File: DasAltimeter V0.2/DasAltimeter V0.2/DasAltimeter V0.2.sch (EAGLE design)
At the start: 53 parts, among them IC1 BMI055, U1 ATSAMD21G-A, U2 3.3V/150mA, U3 MS5803-14BA, U4 ADXL193, X1 22-23-2041, X2 22-23-2041

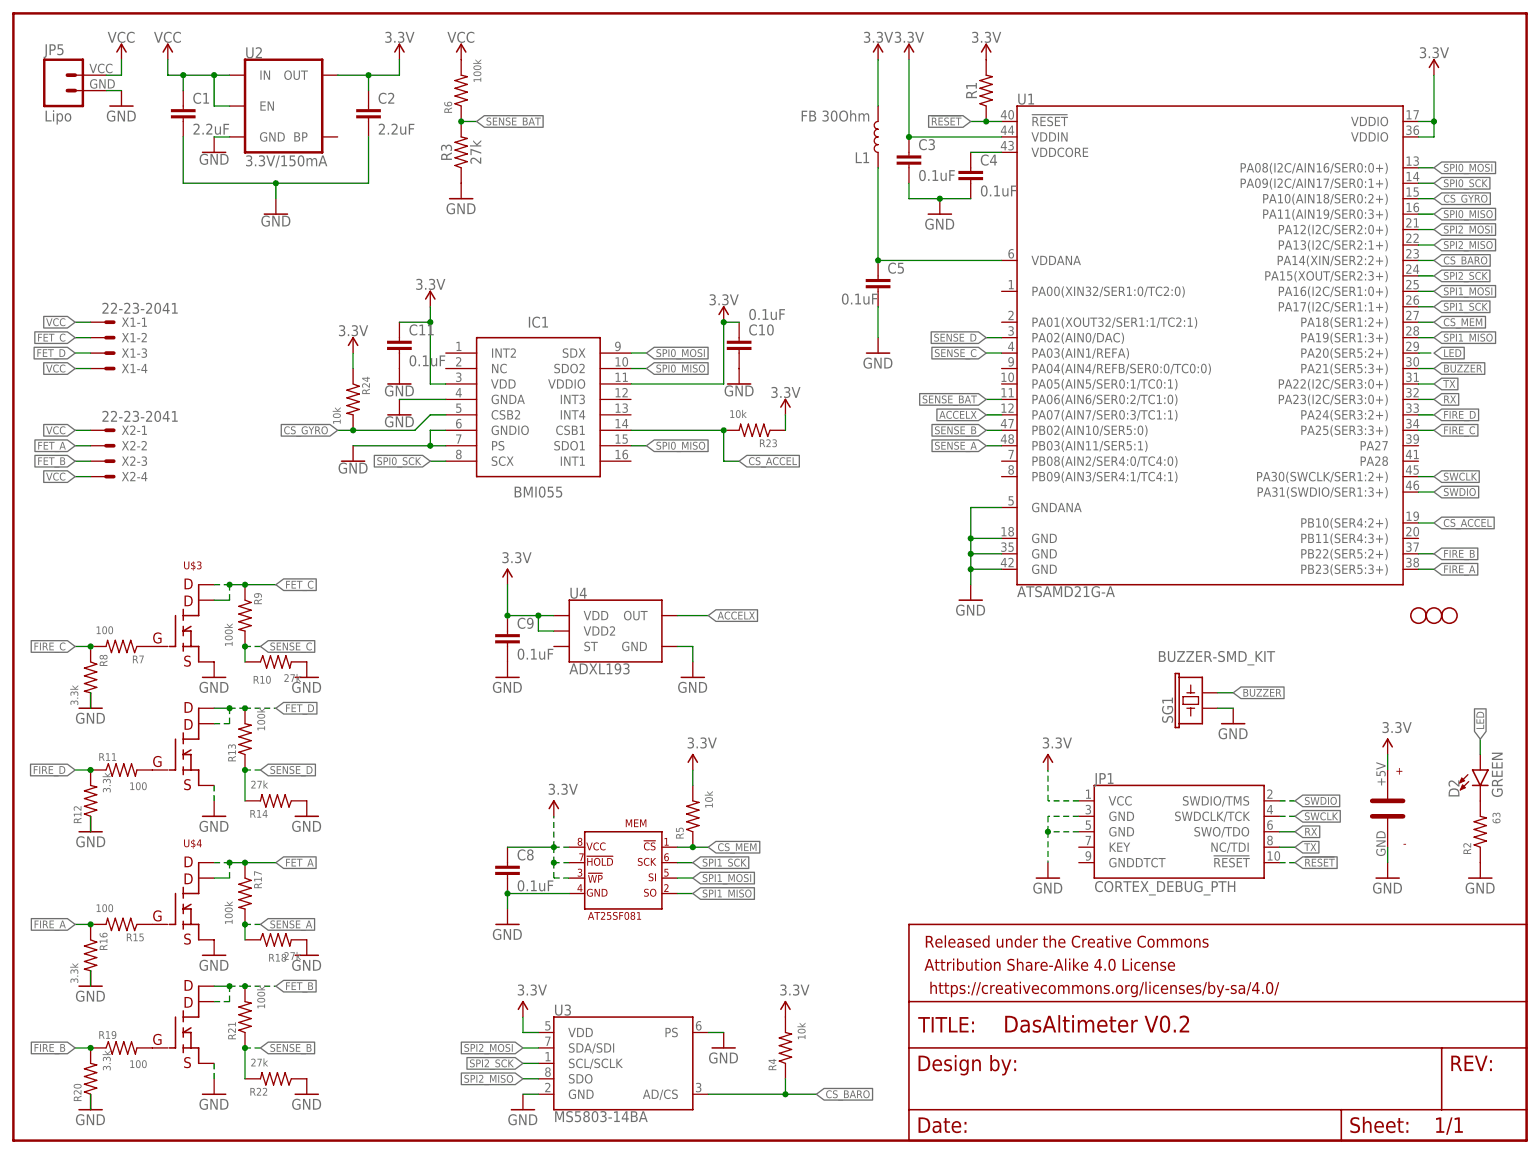
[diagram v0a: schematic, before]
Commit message: playing with mini altimeter idea
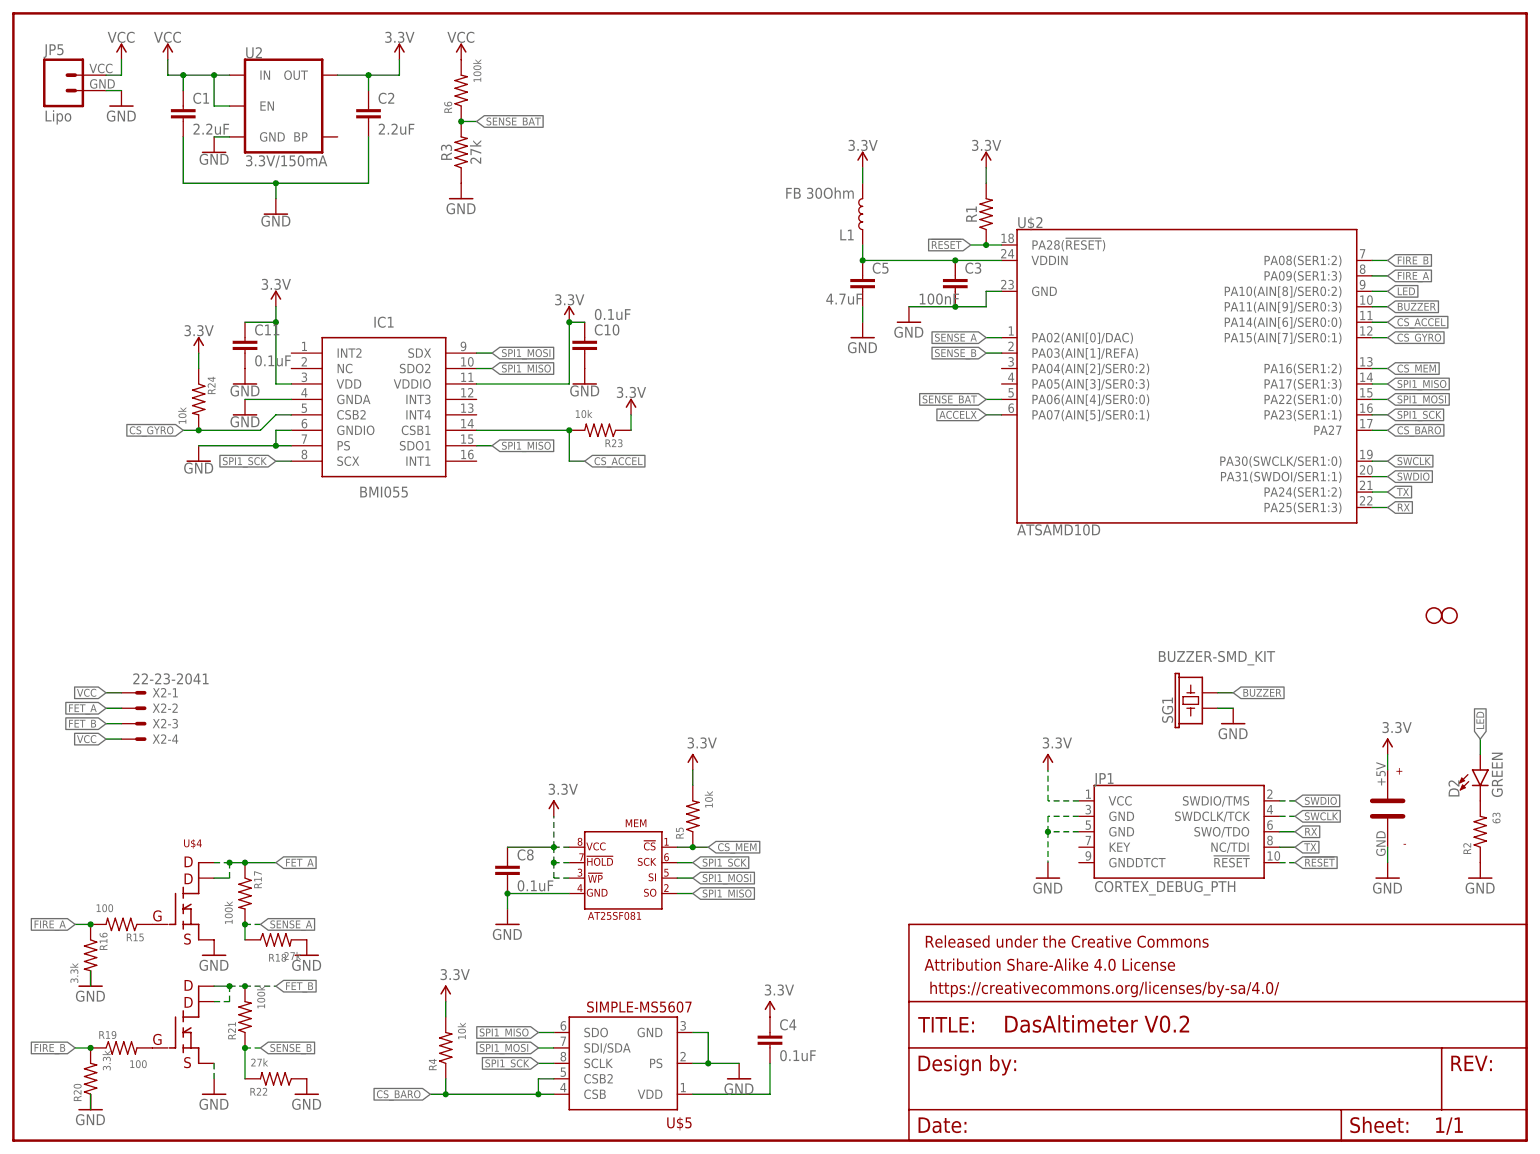
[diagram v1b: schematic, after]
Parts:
- removed C9: 0.1uF, SparkFun-Capacitors:0.1UF-0402-16V-10%
- removed H1: STAND-OFFTIGHT, SparkFun-Hardware:STAND-OFFTIGHT
- removed R10, R14: 27k, SparkFun-Resistors:RESISTOR0402
- removed R11, R7: 100, SparkFun-Resistors:RESISTOR0402
- removed R12, R8: 3.3k, SparkFun-Resistors:RESISTOR0402
- removed R13, R9: 100k, SparkFun-Resistors:RESISTOR0402
- removed U$3: SI7232DN, SaL-lib1:SI7232DN
- removed U1: ATSAMD21G-A, SparkFun-IC-Microcontroller:ATSAMD21G-A
- removed U3: MS5803-14BA, SparkFun-Sensors:MS5803-14BA
- removed U4: ADXL193, SparkFun-Sensors:ADXL193
- removed X1: 22-23-2041, con-molex:22-23-2041
- added U$2: ATSAMD10D, SaL-lib1:ATSAMD10D
- added U$5: SIMPLE-MS5607, MS5607:SIMPLE-MS5607
- C3: value 0.1uF -> 100nF
- C5: value 0.1uF -> 4.7uF
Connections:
- removed net FET_C: R9.1, U$3.PIN7, U$3.PIN8, X1-2.S
- removed net FET_D: R13.2, U$3.PIN5, U$3.PIN6, X1-3.S
- removed net FIRE_C: R7.2, R8.1, U1.PA25(SER3:3+)
- removed net FIRE_D: R11.1, R12.2, U1.PA24(SER3:2+)
- removed net N$3: C4.1, U1.VDDCORE
- removed net N$8: R11.2, U$3.PIN4
- removed net SENSE_C: R10.1, R9.2, U1.PA03(AIN1/REFA)
- removed net SENSE_D: R13.1, R14.2, U1.PA02(AIN0/DAC)
- removed net SPI0_MISO: IC1.SDO1, IC1.SDO2, U1.PA11(AIN19/SER0:3+)
- removed net SPI0_MOSI: IC1.SDX, U1.PA08(I2C/AIN16/SER0:0+)
- removed net SPI0_SCK: IC1.SCX, U1.PA09(I2C/AIN17/SER0:1+)
- removed net SPI2_MISO: U1.PA13(I2C/SER2:1+), U3.SDO
- removed net SPI2_MOSI: U1.PA12(I2C/SER2:0+), U3.SDA/SDI
- removed net SPI2_SCK: U1.PA15(XOUT/SER2:3+), U3.SCL/SCLK
- net !RESET: now also U$2.PA28(!RESET!); no longer U1.!RESET!
- net 3.3V: now also C4.1; no longer C3.1, C9.1, U1.VDDIN, U1.VDDIO@17, U1.VDDIO@36, U3.VDD, U4.VDD, U4.VDD2
- net ACCELX: now also U$2.PA07(AIN[5]/SER0:1); no longer U1.PA07(AIN7/SER0:3/TC1:1), U4.OUT
- net BUZZER: now also U$2.PA11(AIN[9]/SER0:3); no longer U1.PA21(SER5:3+)
- net CS_ACCEL: now also U$2.PA14(AIN[6]/SER0:0); no longer U1.PB10(SER4:2+)
- net CS_BARO: now also U$2.PA27, U$5.CSB2; no longer U1.PA14(XIN/SER2:2+), U3.AD/CS
- net CS_GYRO: now also U$2.PA15(AIN[7]/SER0:1); no longer U1.PA10(AIN18/SER0:2+)
- net CS_MEM: now also U$2.PA16(SER1:2); no longer U1.PA18(SER1:2+)
- net FIRE_A: now also U$2.PA09(SER1:3); no longer U1.PB23(SER5:3+)
- net FIRE_B: now also U$2.PA08(SER1:2); no longer U1.PB22(SER5:2+)
- net GND: now also U$2.GND@23, U$5.GND; no longer C4.2, C9.2, R10.2, R12.1, R14.1, R8.2, U$3.PIN1, U$3.PIN3, U1.GND@18, U1.GND@35, U1.GND@42, U1.GNDANA, U3.GND, U3.PS, U4.GND
- net LED: now also U$2.PA10(AIN[8]/SER0:2); no longer U1.PA20(SER5:2+)
- net N$1: now also C4.2, U$5.VDD; no longer R7.1, U$3.PIN2
- net N$4: now also C3.1, U$2.VDDIN; no longer U1.VDDANA
- net RX: now also U$2.PA25(SER1:3); no longer U1.PA23(I2C/SER3:0+)
- net SENSE_A: now also U$2.PA02(ANI[0]/DAC); no longer U1.PB03(AIN11/SER5:1)
- net SENSE_B: now also U$2.PA03(AIN[1]/REFA); no longer U1.PB02(AIN10/SER5:0)
- net SENSE_BAT: now also U$2.PA06(AIN[4]/SER0:0); no longer U1.PA06(AIN6/SER0:2/TC1:0)
- net SPI1_MISO: now also IC1.SDO1, IC1.SDO2, U$2.PA17(SER1:3); no longer U1.PA19(SER1:3+)
- net SPI1_MOSI: now also IC1.SDX, U$2.PA22(SER1:0); no longer U1.PA16(I2C/SER1:0+)
- net SPI1_SCK: now also IC1.SCX, U$2.PA23(SER1:1); no longer U1.PA17(I2C/SER1:1+)
- net SWCLK: now also U$2.PA30(SWCLK/SER1:0); no longer U1.PA30(SWCLK/SER1:2+)
- net SWDIO: now also U$2.PA31(SWDOI/SER1:1); no longer U1.PA31(SWDIO/SER1:3+)
- net TX: now also U$2.PA24(SER1:2); no longer U1.PA22(I2C/SER3:0+)
- net VCC: no longer X1-1.S, X1-4.S
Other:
- moved on the sheet: C10, C11, C3, C4, C5, IC1, L1, R1, R23, R24, R4, X2-1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
